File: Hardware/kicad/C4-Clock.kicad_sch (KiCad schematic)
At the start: 24 parts, among them J1 Keypad, J2 Battery, J3 LCD1602, J4 Boost Module, K1 FINDER-36.11-5V, Q1 S9014, Q2 S9014, SW1 SW_SPST, SW2 SW_SPST, U1 ATmega328P-P, U2 AMS1117-5.0, U3 PCF8574A, Y1 16MHz

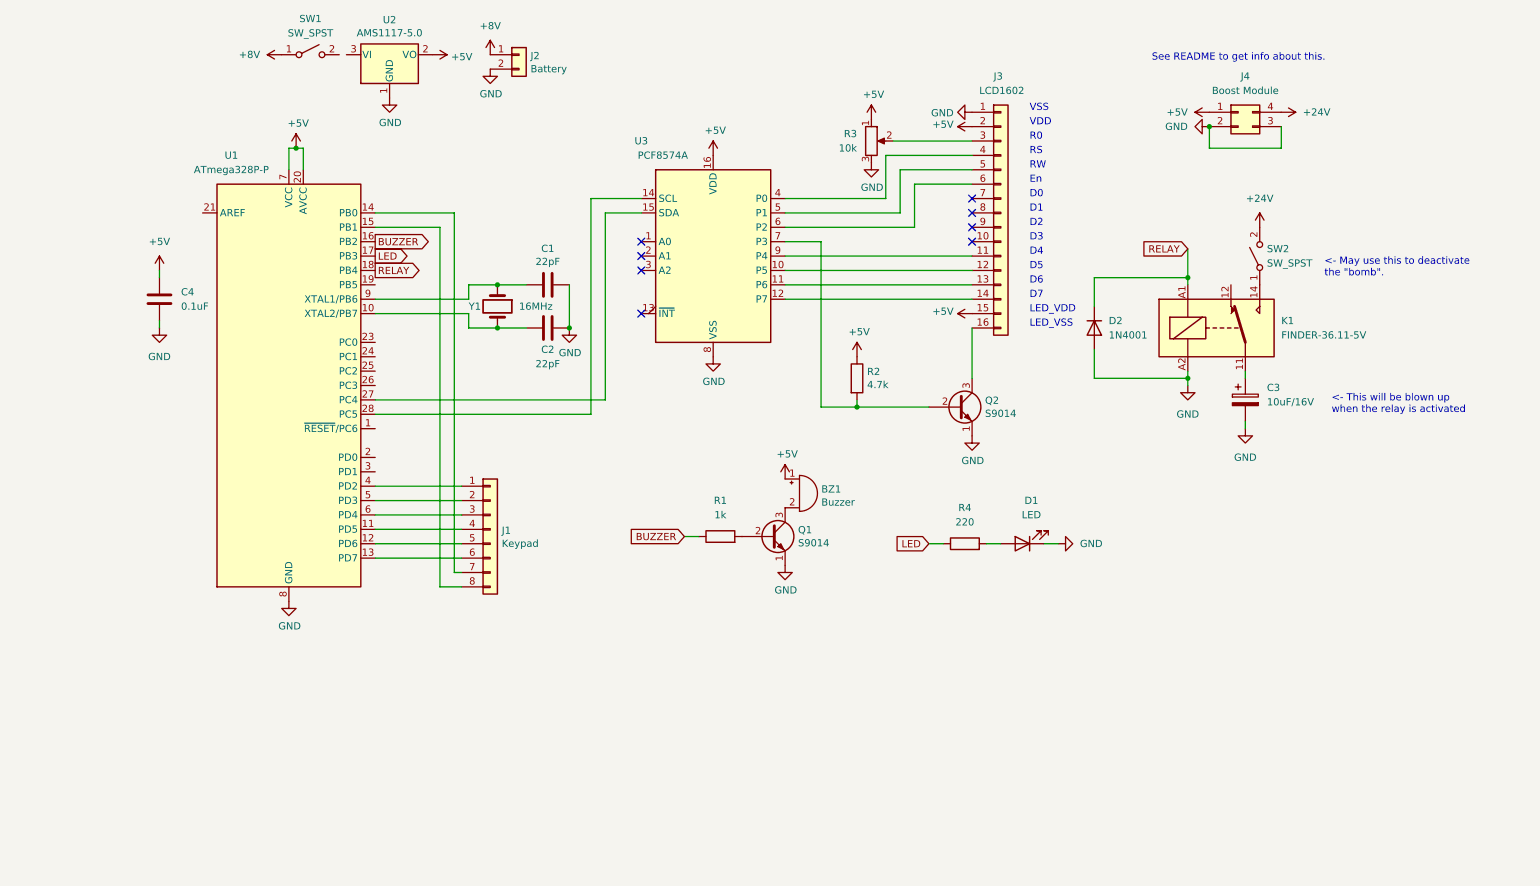
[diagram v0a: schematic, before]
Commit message: kicad: create PCB
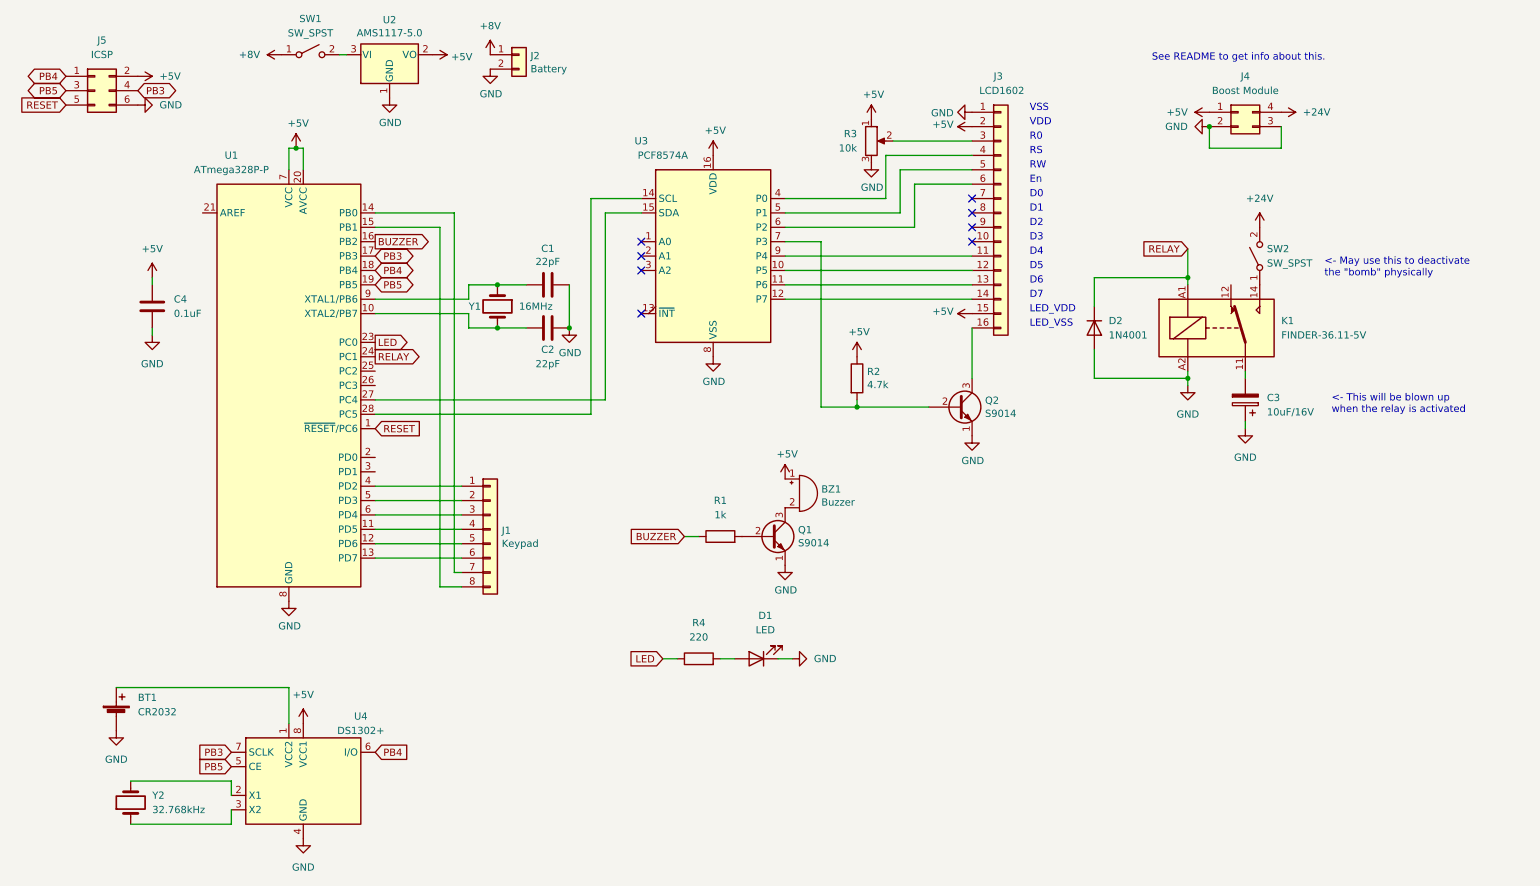
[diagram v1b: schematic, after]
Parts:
- added BT1: CR2032, Battery:BatteryHolder_ComfortableElectronic_CH273-2450_1x2450, symbol Device:Battery_Cell
- added J5: ICSP, Connector_PinHeader_2.54mm:PinHeader_2x03_P2.54mm_Vertical, symbol Connector_Generic:Conn_02x03_Odd_Even
- added U4: DS1302+, Package_DIP:DIP-8_W7.62mm, symbol Timer_RTC:DS1302+
- added Y2: 32.768kHz, Crystal:Crystal_AT310_D3.0mm_L10.0mm_Horizontal, symbol Device:Crystal
- BZ1: footprint (none) -> Buzzer_Beeper:Buzzer_12x9.5RM7.6
- C1, C2: footprint Capacitor_THT:C_Disc_D3.0mm_W1.6mm_P2.50mm -> Capacitor_THT:C_Disc_D4.3mm_W1.9mm_P5.00mm
- C4: footprint (none) -> Capacitor_THT:C_Disc_D4.3mm_W1.9mm_P5.00mm
- D1: footprint (none) -> LED_THT:LED_D5.0mm
- D2: footprint (none) -> Diode_THT:D_A-405_P7.62mm_Horizontal
- J4: footprint (none) -> DC-Buck:DC-Buck-2A
- R3: footprint Resistor_THT:R_Axial_DIN0207_L6.3mm_D2.5mm_P10.16mm_Horizontal -> Potentiometer_THT:Potentiometer_Vishay_T73YP_Vertical
- SW2: footprint Button_Switch_THT:SW_E-Switch_EG1271_DPDT -> Button_Switch_THT:SW_Push_2P2T_Toggle_CK_PVA2xxH1xxxxxxV2
- U1: footprint Package_DIP:DIP-28_W7.62mm -> Package_DIP:DIP-28_W7.62mm_Socket
- Y1: footprint (none) -> Crystal:Crystal_HC49-4H_Vertical
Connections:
- net +5V: now also J5.2 (Pin_2), U4.8 (VCC1)
- net GND: now also C3.1, BT1.2 (-), J5.6 (Pin_6), U4.4 (GND); no longer C3.2
- net LED: now also U1.23 (PC0); no longer U1.17 (PB3)
- net RELAY: now also U1.24 (PC1); no longer U1.18 (PB4)
- net at U2.3 (VI): now also SW1.2 (B)
- net RESET: now reaches U1.1 (~{RESET}/PC6)
- net RESET: now also J5.5 (Pin_5)
- net PB5: now reaches U1.19 (PB5)
- net PB5: now also J5.3 (Pin_3), U4.5 (CE)
- net at K1.11: now also C3.2; no longer C3.1
- new net: BT1.1 (+), U4.1 (VCC2)
- new net: U4.2 (X1), Y2.2
- new net: U4.3 (X2), Y2.1
- new net PB3: J5.4 (Pin_4), U1.17 (PB3), U4.7 (SCLK)
- new net PB4: J5.1 (Pin_1), U1.18 (PB4), U4.6 (I/O)
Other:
- note added: "<- May use this to deactivate the "bomb" physically"
- note removed: "<- May use this to deactivate the "bomb"."
- moved on the sheet: C3, C4, D1, R4
